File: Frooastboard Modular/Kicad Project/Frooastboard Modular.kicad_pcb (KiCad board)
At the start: 4 copper layers, 44.6 x 25.7 mm, 41 parts, among them J1 Conn_01x16, J2 Conn_01x06, J3 Conn_01x06, J4 Conn_01x10, J5 Conn_01x12, J6 SW Interface, J7 Conn_01x04, U1 IS31FL3733-QF, U2 RP2040, U3 W25Q32JVZP, U4 LM317L_SOT-89, Y1 12MHz

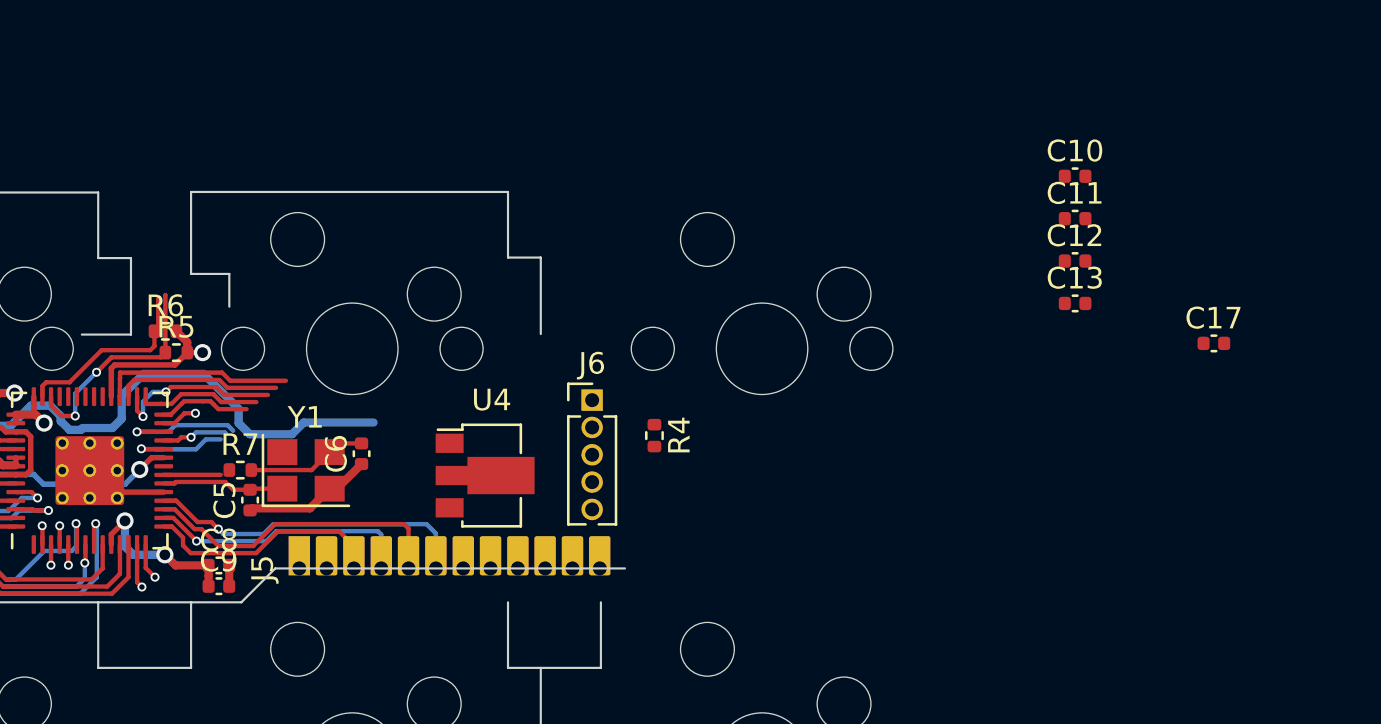
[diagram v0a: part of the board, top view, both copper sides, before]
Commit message: Update Frooastboard Modular.kicad_pcb
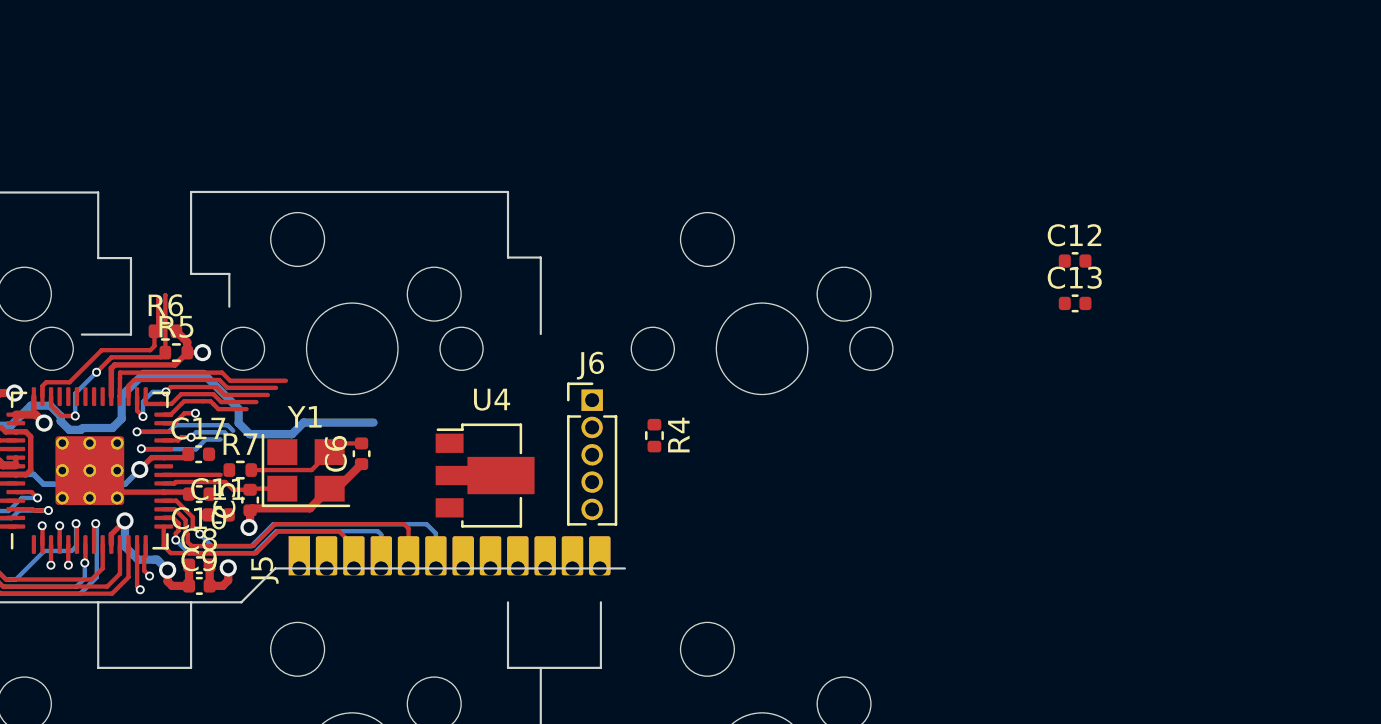
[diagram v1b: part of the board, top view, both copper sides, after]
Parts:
- moved C17 47.5 mm to (63.9, 62.7)
- moved C10 43.3 mm to (63.9, 64.6), turned to 180 degrees
- moved C11 42.1 mm to (64.8, 65.5)
- moved C8 0.91 mm to (63.9, 67.9)
- moved C9 0.91 mm to (63.9, 68.8)
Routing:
- net GND: track 32.8 -> 36.4 mm, vias 4 -> 6
- net Net-(J5-Pin_4): track 12.4 -> 13.9 mm
- net +1V1: track 17.2 -> 18.4 mm
- net Net-(J5-Pin_6): track 15.3 -> 16.0 mm
- net Net-(J5-Pin_5): track 14.4 -> 15.0 mm
